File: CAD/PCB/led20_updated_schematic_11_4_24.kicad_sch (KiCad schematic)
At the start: 33 parts, among them U6 B2B-PH-K-S, U7 B2B-PH-K-S

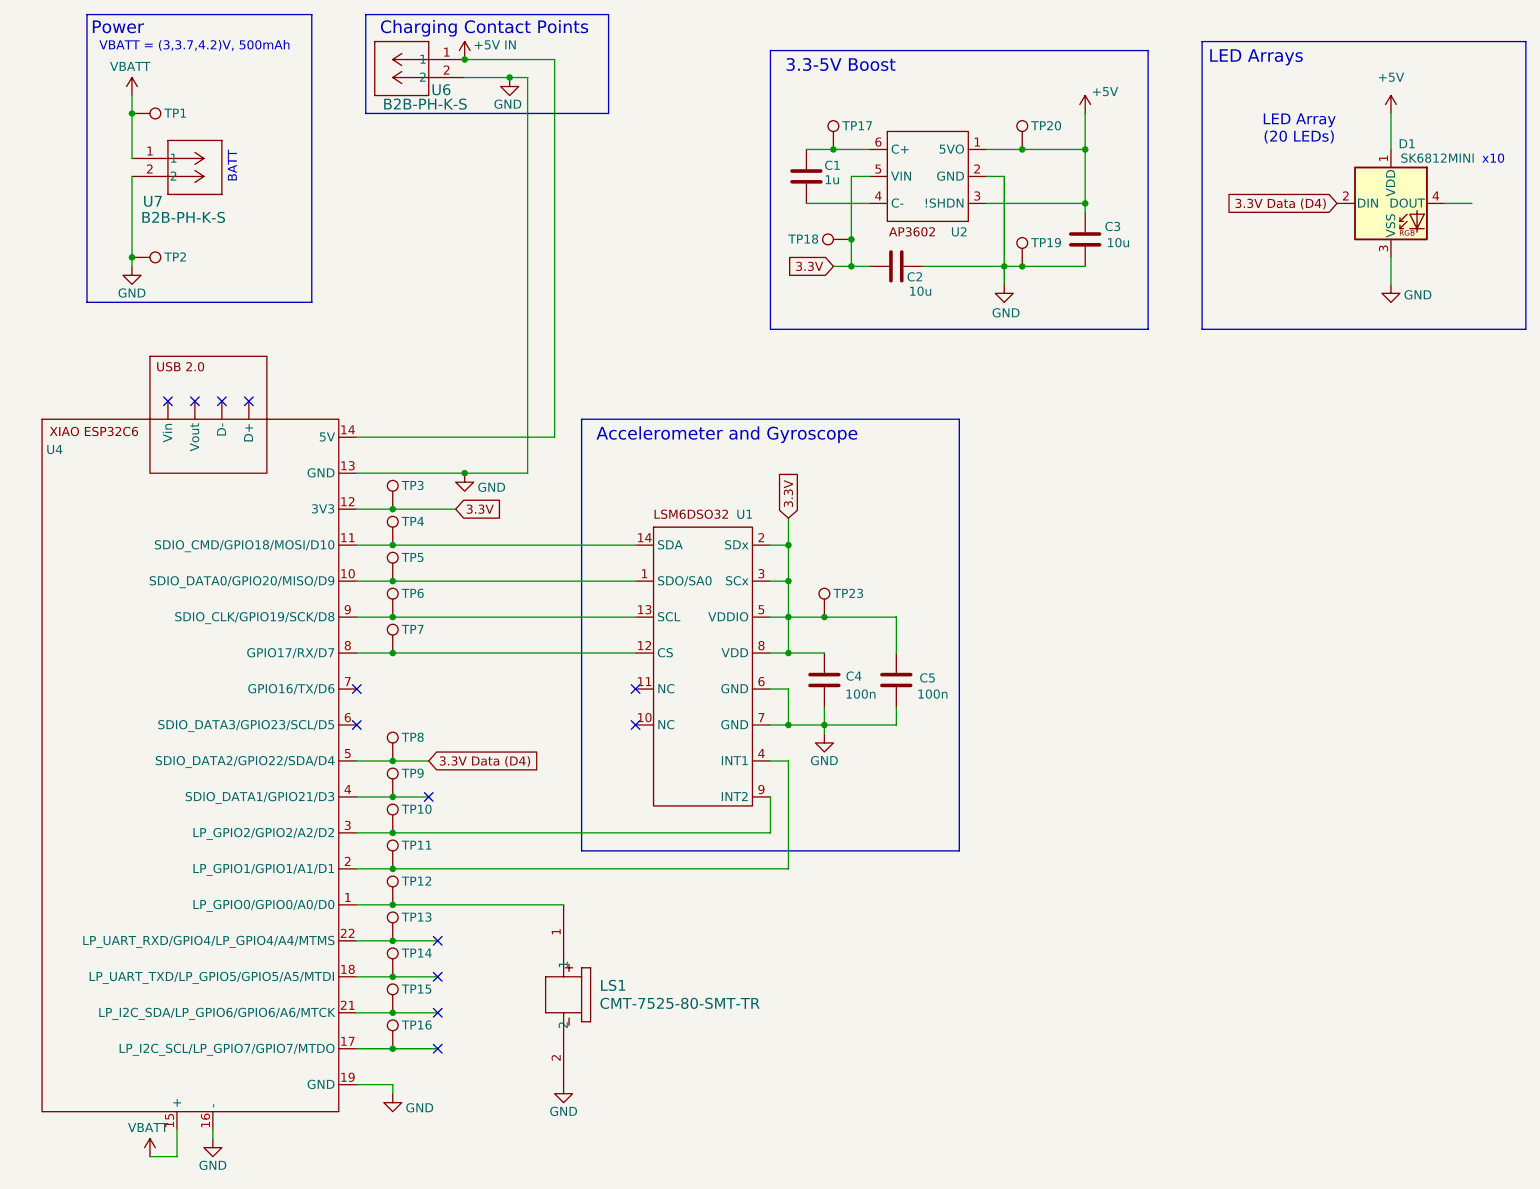
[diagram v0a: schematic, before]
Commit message: PCB
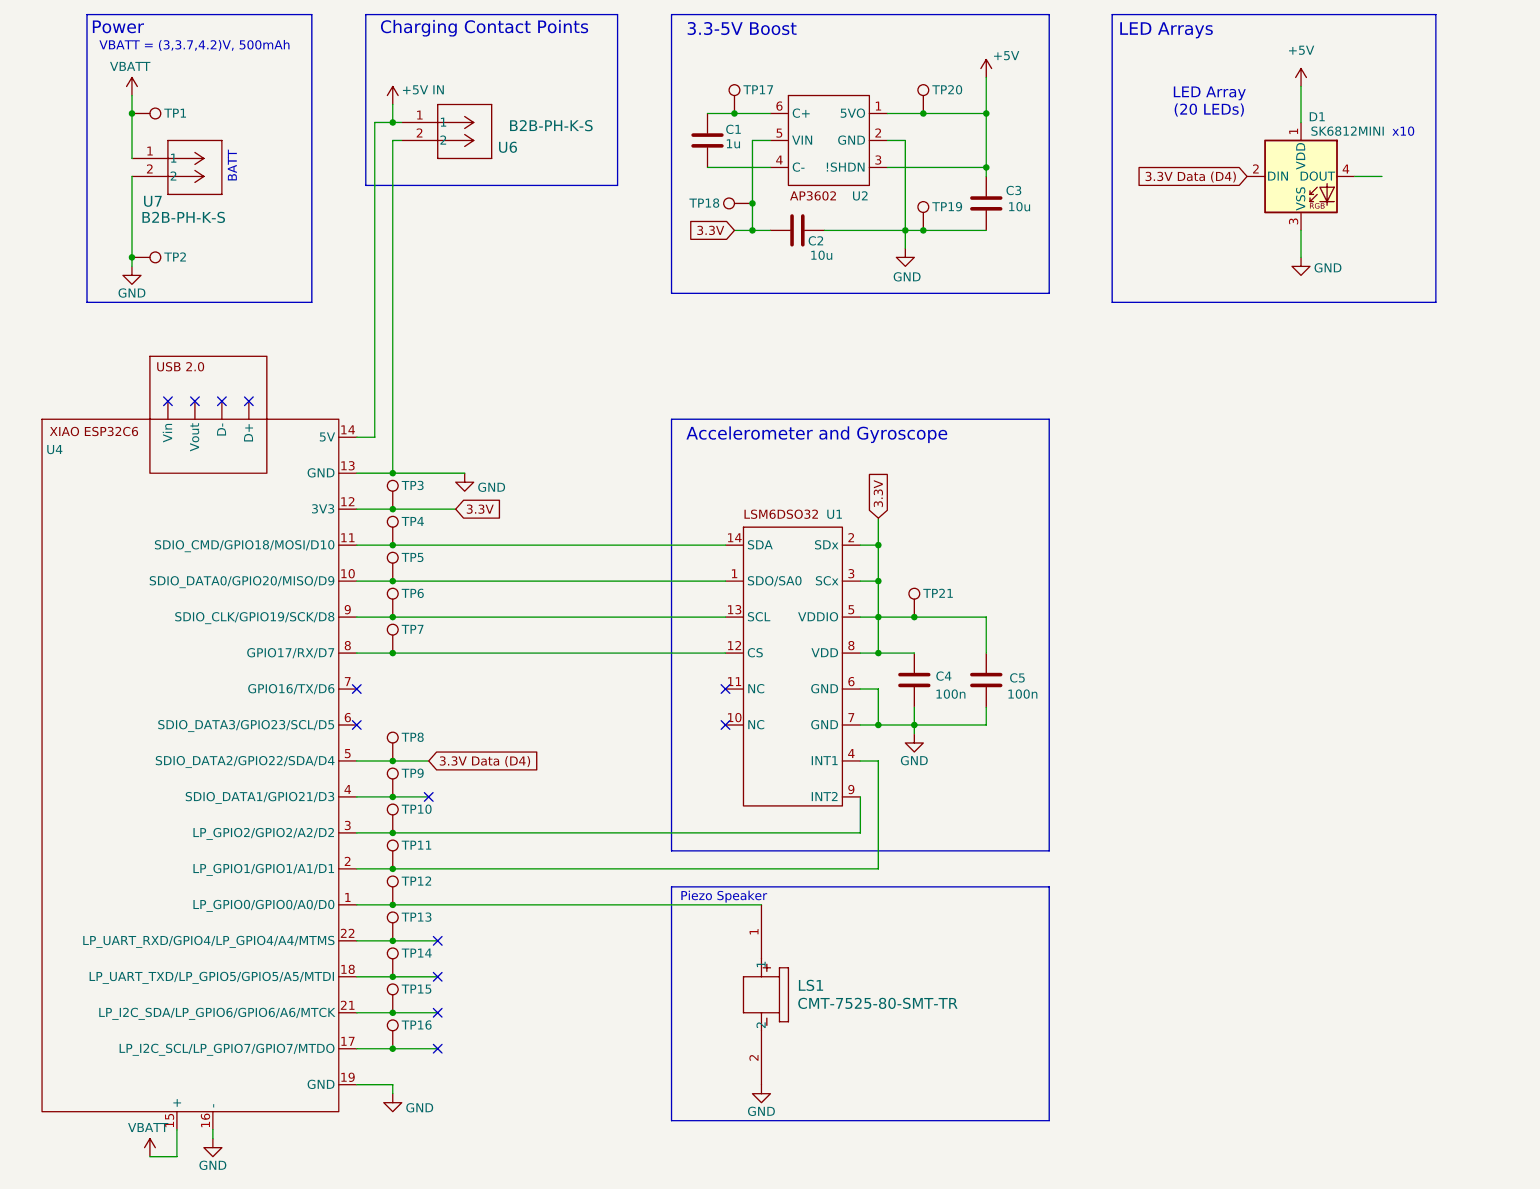
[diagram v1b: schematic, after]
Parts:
- renumbered TP23 to TP21
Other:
- note added: "Piezo Speaker"
- moved on the sheet: C1, C2, C3, C4, C5, D1, LS1, TP17, TP18, TP19, TP20, TP21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
